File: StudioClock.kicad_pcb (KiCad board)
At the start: 2 copper layers, 80 parts, among them J1 CONN_01X16, J2 CONN_01X16, U1 7SEGMENTS, U2 7SEGMENTS, U3 7SEGMENTS, U4 7SEGMENTS

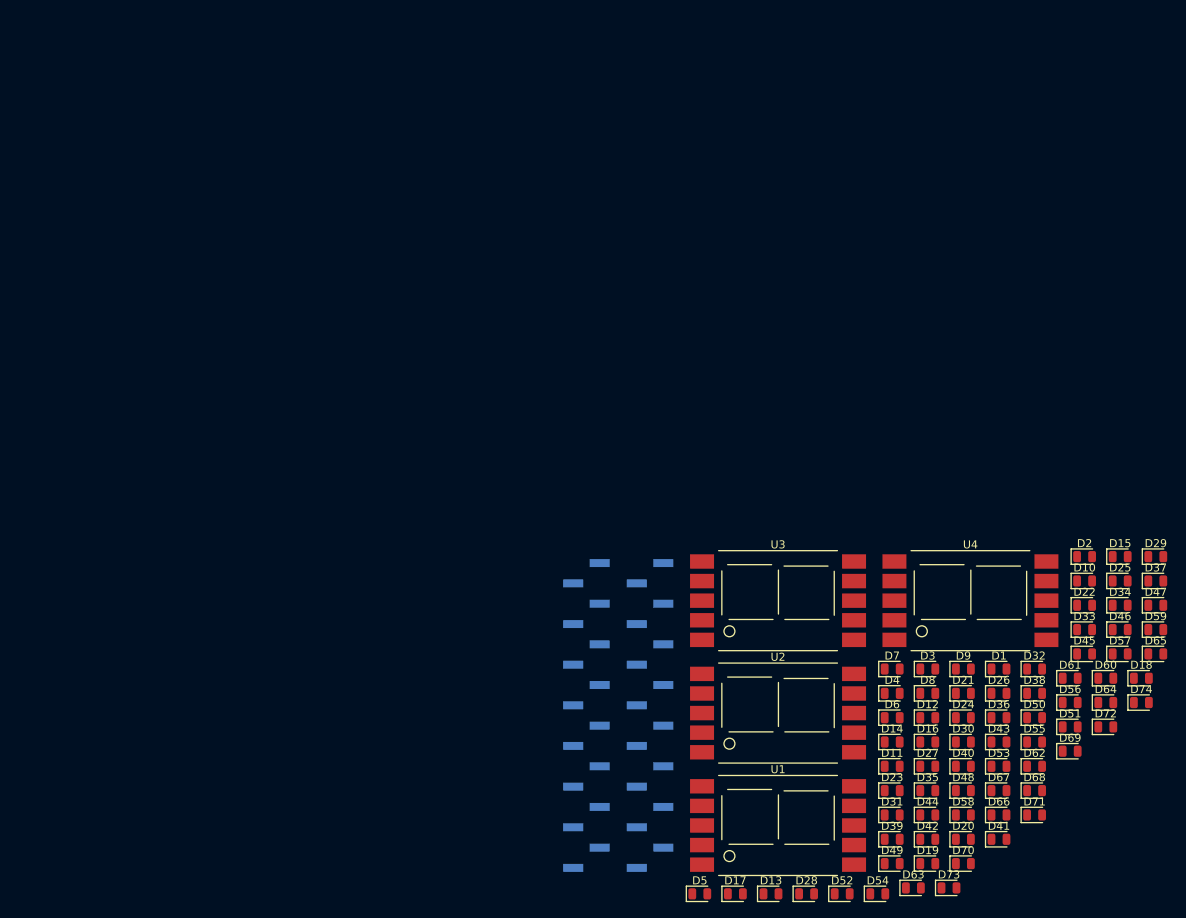
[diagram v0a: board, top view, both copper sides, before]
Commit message: executed and cleaned up files, added README
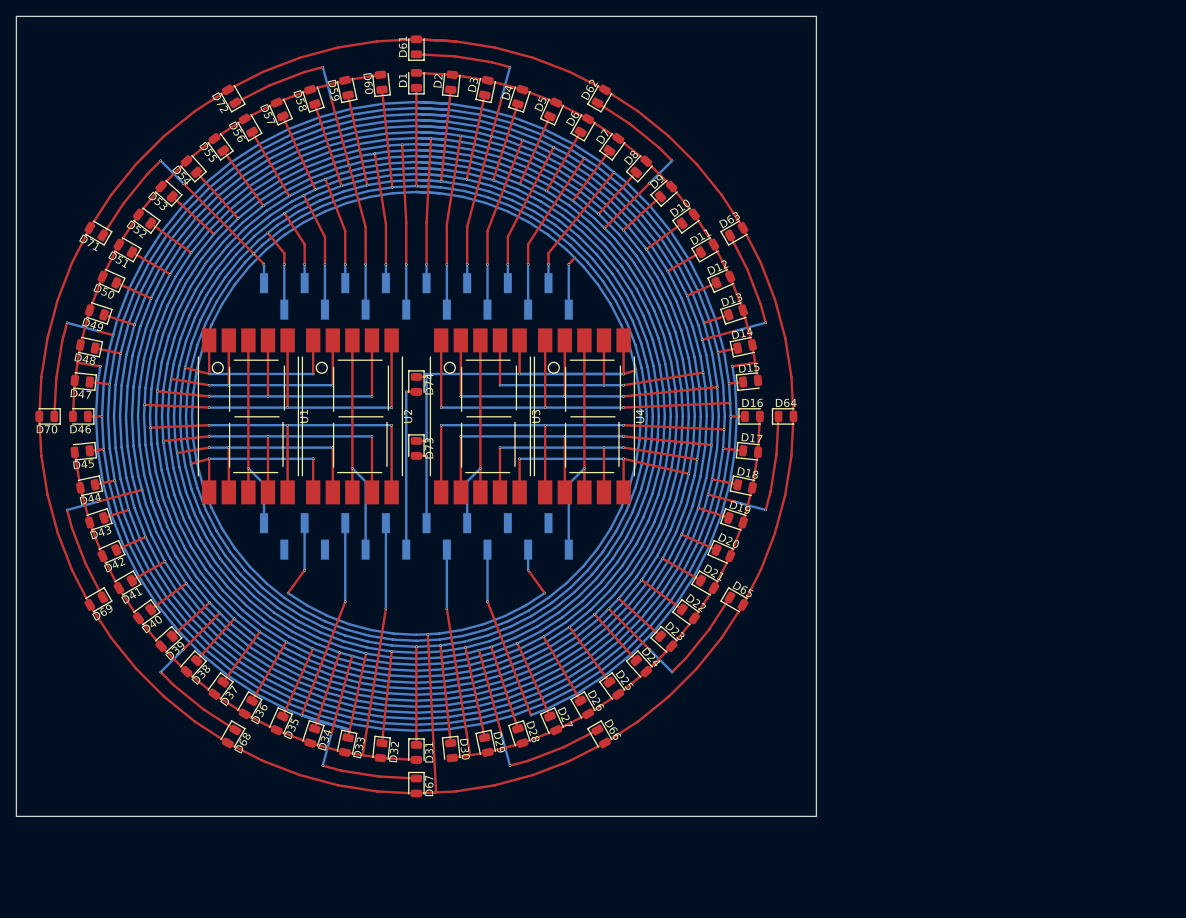
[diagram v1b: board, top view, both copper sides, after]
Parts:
- moved D71 138.1 mm to (-40.0, -23.1), turned to 150 degrees
- moved D47 137.1 mm to (-41.8, -4.39), turned to 174 degrees
- moved D72 134.7 mm to (-23.1, -40.0), turned to 120 degrees
- moved D46 132.7 mm to (-42.0, 0.00), turned to 180 degrees
- moved D51 132.4 mm to (-36.4, -21.0), turned to 150 degrees
- moved D50 127.9 mm to (-38.4, -17.1), turned to 156 degrees
- moved D45 127.8 mm to (-41.8, 4.39), turned to 186 degrees
- moved D70 127.5 mm to (-46.2, 0.00), turned to 180 degrees
- moved D53 126.4 mm to (-31.2, -28.1), turned to 138 degrees
- moved D55 126.4 mm to (-24.7, -34.0), turned to 126 degrees
- moved D56 125.5 mm to (-21.0, -36.4), turned to 120 degrees
- moved D57 125.2 mm to (-17.1, -38.4), turned to 114 degrees
- moved D54 125.0 mm to (-28.1, -31.2), turned to 132 degrees
- moved D69 123.2 mm to (-40.0, 23.1), turned to 210 degrees
- moved D48 122.7 mm to (-41.1, -8.73), turned to 168 degrees
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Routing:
- net /a4: track 0.00 -> 370.6 mm, vias 0 -> 5
- net /k14: track 0.00 -> 345.4 mm, vias 0 -> 13
- net /k11: track 0.00 -> 340.0 mm, vias 0 -> 13
- net /k12: track 0.00 -> 338.2 mm, vias 0 -> 13
- net /k7: track 0.00 -> 336.8 mm, vias 0 -> 13
- net /k6: track 0.00 -> 330.7 mm, vias 0 -> 13
- net /k13: track 0.00 -> 329.4 mm, vias 0 -> 10
- net /k9: track 0.00 -> 328.4 mm, vias 0 -> 13
- net /k10: track 0.00 -> 327.1 mm, vias 0 -> 12
- net /k5: track 0.00 -> 325.6 mm, vias 0 -> 12
- net /k8: track 0.00 -> 317.4 mm, vias 0 -> 12
- net /k3: track 0.00 -> 310.7 mm, vias 0 -> 13
- net /k2: track 0.00 -> 303.5 mm, vias 0 -> 13
- net /k4: track 0.00 -> 293.7 mm, vias 0 -> 10
- net /k0: track 0.00 -> 289.2 mm, vias 0 -> 11
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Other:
- board outline added: 100 x 100 mm
